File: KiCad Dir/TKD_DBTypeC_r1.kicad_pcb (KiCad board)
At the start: 2 copper layers, 12 parts, among them J1 JST-SH-SM04B-SRSS-TB

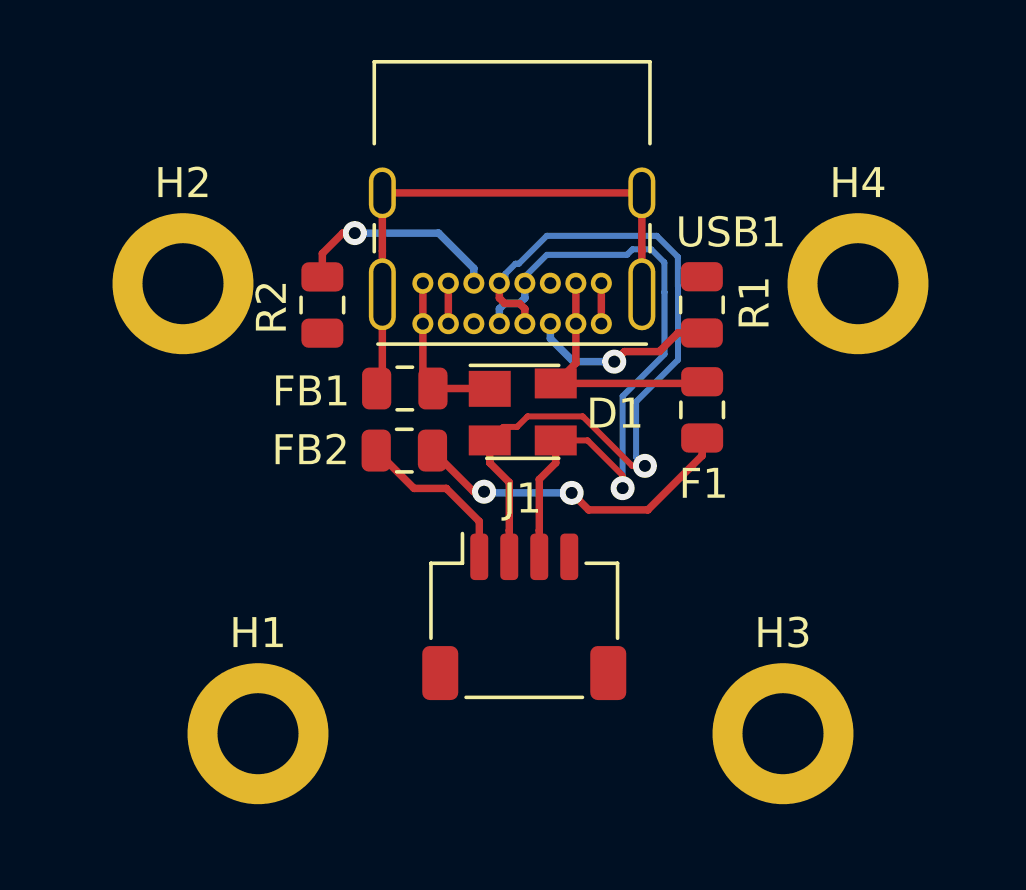
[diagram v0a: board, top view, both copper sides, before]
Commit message: Edge cuts placed, r1 done
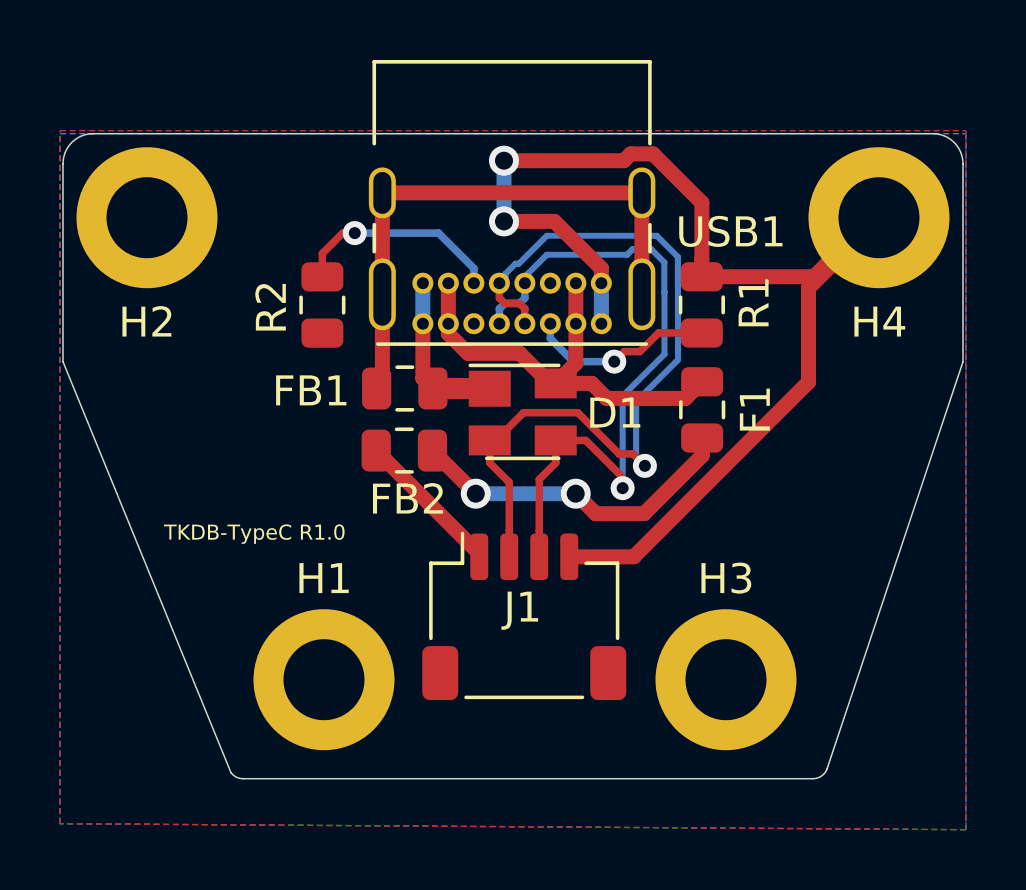
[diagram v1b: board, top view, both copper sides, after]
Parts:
- moved H1 2.84 mm to (59.7, 73.2)
- moved H3 2.62 mm to (73.1, 73.2)
- moved H2 2.51 mm to (53.8, 57.8)
- moved H4 2.31 mm to (78.2, 57.8)
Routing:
- net GND: track 6.90 -> 46.7 mm, vias 0 -> 2
- net VBUS: track 9.87 -> 15.5 mm
- net +5V: track 5.59 -> 5.07 mm
- added copper zone on B.Cu, net GND
- added copper zone on F.Cu, net GND
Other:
- board outline added: 30 x 21.5 mm
- net class POWER added: clearance 0.2, trace_width 0.5, via_dia 1, via_drill 0.6
- board text added: "TKDB-TypeC R1.0"
